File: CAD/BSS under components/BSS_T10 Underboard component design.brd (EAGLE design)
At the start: 23.3 x 22.8 mm, 9 parts, among them IC1 7805DT

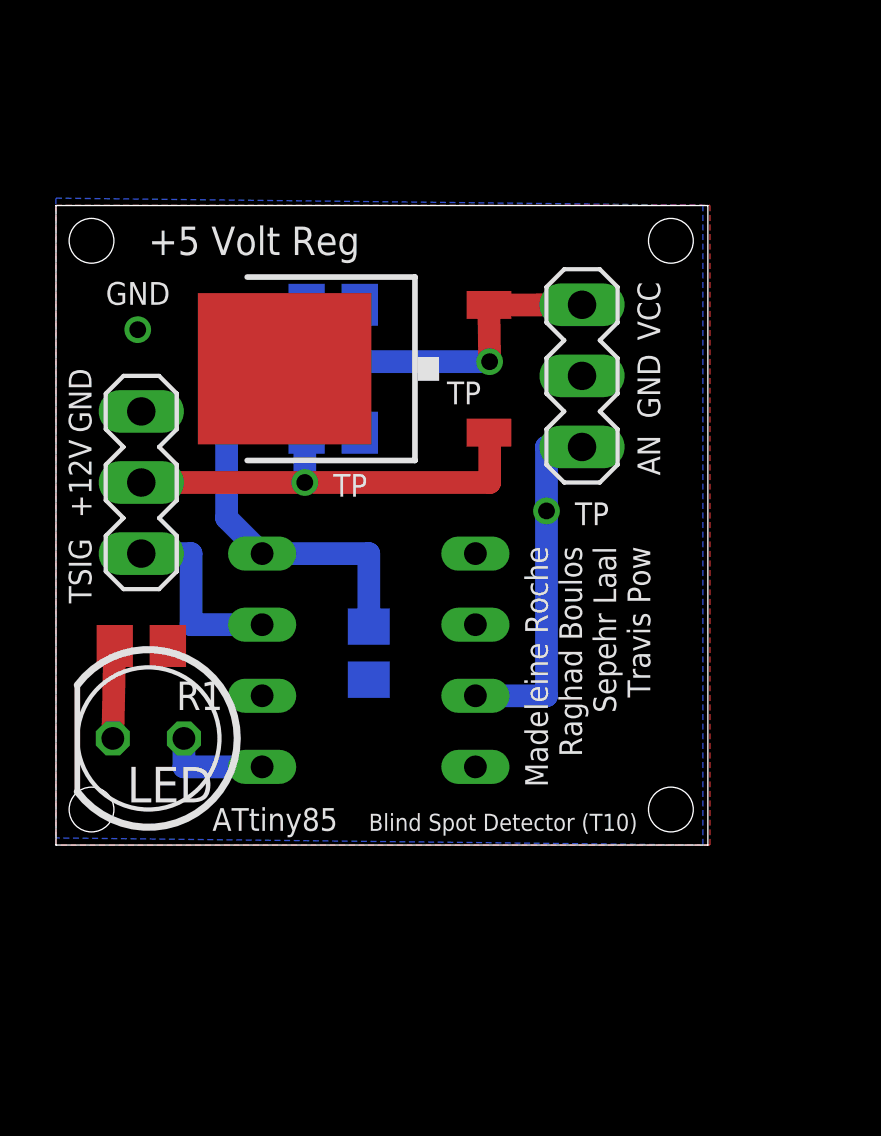
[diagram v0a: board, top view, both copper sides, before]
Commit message: New Board Layout
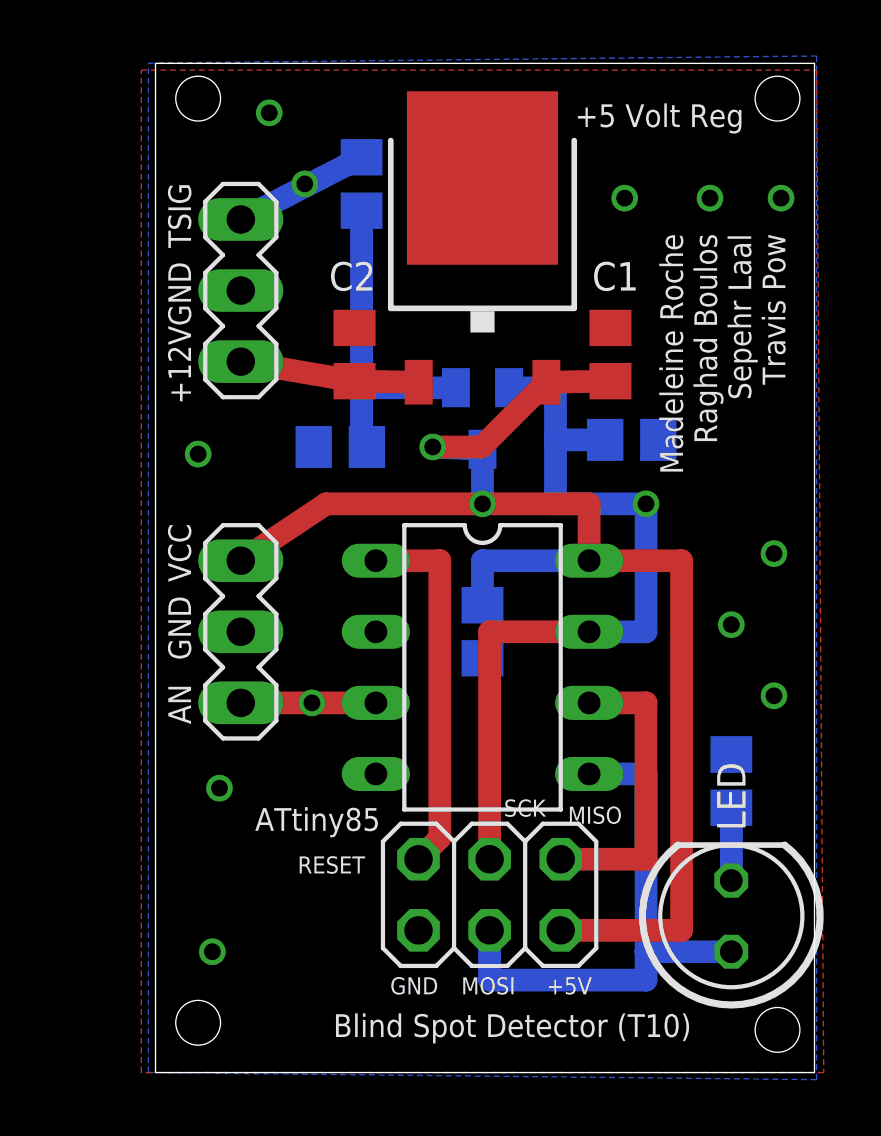
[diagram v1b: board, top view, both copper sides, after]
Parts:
- added JP1: (no value), pinhead:2X03
- added Q1: BSS123, transistor-small-signal:SOT23
- added R2: 10k, rcl:R0805
- added R3: 470k, rcl:R0805
- added R4: 47k, rcl:R0805
- moved LED 21.8 mm to (71.4, 33.0), turned to 90 degrees
- moved R1 21.6 mm to (71.4, 37.8), flipped to the bottom, turned to 270 degrees
- moved TO_SEN 15.2 mm to (53.8, 43.2)
- moved C1 10.1 mm to (67.1, 53.1), flipped to the top, turned to 90 degrees
- moved VOLT_IN 7.73 mm to (53.8, 55.4)
- moved IC1 6.29 mm to (62.5, 56.9), turned to 0 degrees
- moved C3 4.13 mm to (62.5, 43.2)
- moved AVR 4.07 mm to (62.5, 41.9), flipped to the top
- moved C2 2.90 mm to (57.9, 53.1), flipped to the top, turned to 90 degrees
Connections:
- removed net TSIG: AVR.7, VOLT_IN.3
- new net 2N7000: AVR.7, JP1.3, Q1.2, R3.2
- new net N$5: R2.1, VOLT_IN.1
- new net N$6: Q1.1, R2.2, R4.2
- new net N$7: AVR.1, JP1.5
- new net N$9: AVR.6, JP1.1
- net +5V: now also JP1.2, Q1.3
- net 12VBATTERY: now also VOLT_IN.3; no longer VOLT_IN.2
- net GND: now also JP1.6, R3.1, R4.1, VOLT_IN.2; no longer VOLT_IN.1
- net N$4: now also JP1.4
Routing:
- net 2N7000: track 0.00 -> 29.1 mm, vias 0 -> 1
- net +5V: track 33.4 -> 52.4 mm, vias 1 -> 2
- net N$4: track 3.81 -> 19.8 mm
- net N$7: track 0.00 -> 13.3 mm
- net N$6: track 0.00 -> 12.0 mm
- net N$9: track 0.00 -> 10.7 mm
- net 12VBATTERY: track 16.1 -> 6.42 mm, vias 1 -> 0
- net N$1: track 12.7 -> 4.83 mm
- net TSIG: track 6.86 -> 0.00 mm
- net N$5: track 0.00 -> 4.86 mm
- net RLED: track 3.30 -> 2.61 mm
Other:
- board size 23.3 x 22.8 mm -> 23.5 x 36.1 mm
- board text added: "+5V"
- board text added: "2N7000"
- board text added: "MISO"
- board text added: "MOSI"
- board text added: "RESET"
- board text added: "SCK"
- board text removed: "TP"
